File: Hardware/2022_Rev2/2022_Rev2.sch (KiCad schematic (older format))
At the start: 36 parts

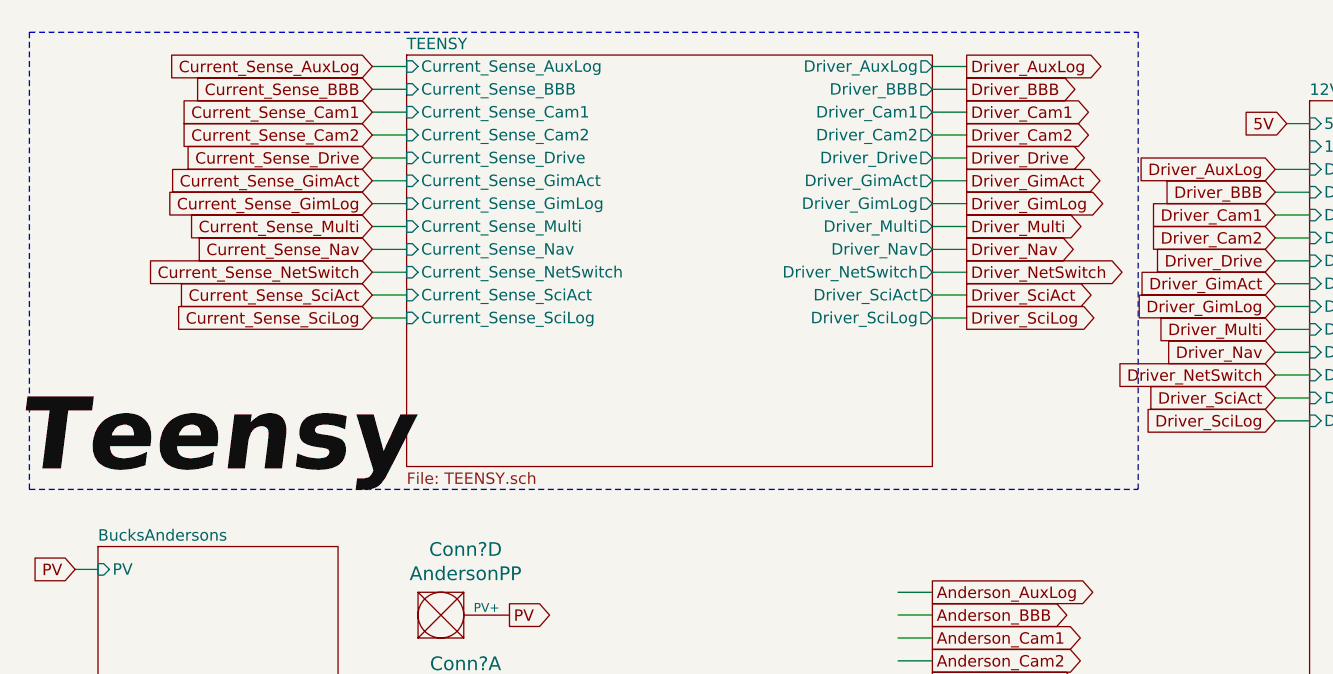
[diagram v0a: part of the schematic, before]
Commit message: molex pins
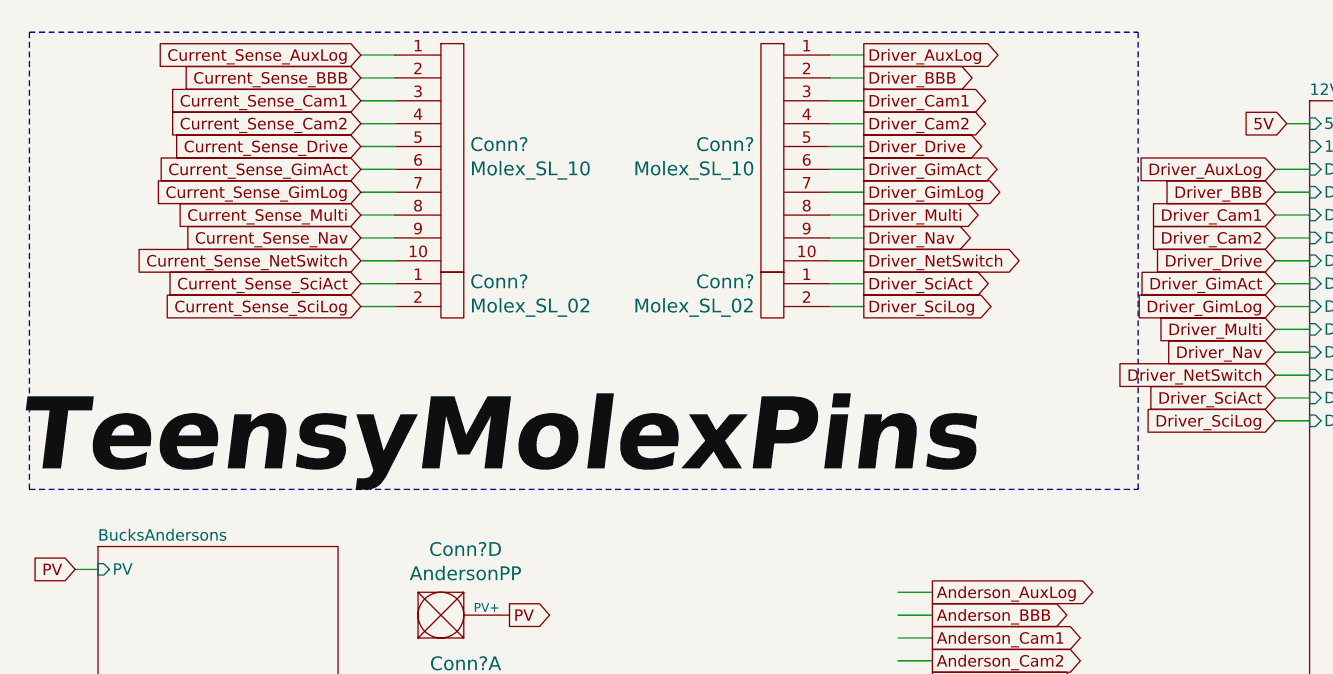
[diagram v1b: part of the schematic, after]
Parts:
- added Conn? (x2): Molex_SL_10, symbol MRDT_Connectors:Molex_SL_10
- added Conn? (x2): Molex_SL_02, symbol MRDT_Connectors:Molex_SL_02
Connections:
- net labels added: TeensyMolexPins
- net labels removed: Teensy
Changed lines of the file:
@@
 $Descr A4 11693 8268
 encoding utf-8
-Sheet 1 5
+Sheet 1 4
 Title ""
 Date ""
@@
 	1    0    0    -1
 $EndComp
-Text GLabel 2000 1050 0    50   Input ~ 0
-Current_Sense_Drive
-Text GLabel 2000 1450 0    50   Input ~ 0
-Current_Sense_Nav
-Wire Wire Line
-	2000 1050 2150 1050
-Wire Wire Line
-	2150 1450 2000 1450
-Text GLabel 4600 1050 2    50   Output ~ 0
-Driver_Drive
-Wire Wire Line
-	4450 1050 4600 1050
-Text GLabel 4600 1450 2    50   Output ~ 0
-Driver_Nav
-Wire Wire Line
-	4450 1450 4600 1450
 Wire Notes Line
 	500  500  5350 500
 Text Label 450  2500 0    315  Italic 63
-Teensy
+TeensyMolexPins
 Wire Notes Line
 	500  2500 5350 2500
@@
 Text Label 7100 7050 0    157  Italic 31
 "Rev4"
-$Sheet
-S 2150 600  2300 1800
-U 62118F7B
-F0 "TEENSY" 50
-F1 "TEENSY.sch" 50
-F2 "Current_Sense_Drive" I L 2150 1050 50
-F3 "Current_Sense_Nav" I L 2150 1450 50
-F4 "Driver_Drive" O R 4450 1050 50
-F5 "Driver_Nav" O R 4450 1450 50
-F6 "Current_Sense_BBB" I L 2150 750 50
-F7 "Current_Sense_Multi" I L 2150 1350 50
-F8 "Current_Sense_Cam2" I L 2150 950 50
-F9 "Current_Sense_Cam1" I L 2150 850 50
-F10 "Driver_BBB" O R 4450 750 50
-F11 "Driver_Multi" O R 4450 1350 50
-F12 "Driver_GimAct" O R 4450 1150 50
-F13 "Driver_Cam1" O R 4450 850 50
-F14 "Driver_Cam2" O R 4450 950 50
-F15 "Current_Sense_GimAct" I L 2150 1150 50
-F16 "Driver_GimLog" O R 4450 1250 50
-F17 "Driver_NetSwitch" O R 4450 1550 50
-F18 "Driver_AuxLog" O R 4450 650 50
-F19 "Driver_SciLog" O R 4450 1750 50
-F20 "Driver_SciAct" O R 4450 1650 50
-F21 "Current_Sense_GimLog" I L 2150 1250 50
-F22 "Current_Sense_NetSwitch" I L 2150 1550 50
-F23 "Current_Sense_SciAct" I L 2150 1650 50
-F24 "Current_Sense_SciLog" I L 2150 1750 50
-F25 "Current_Sense_AuxLog" I L 2150 650 50
-$EndSheet
-Text GLabel 2000 650  0    50   Input ~ 0
-Current_Sense_AuxLog
-Wire Wire Line
-	2000 650  2150 650
-Text GLabel 2000 750  0    50   Input ~ 0
-Current_Sense_BBB
-Wire Wire Line
-	2000 750  2150 750
-Text GLabel 2000 850  0    50   Input ~ 0
-Current_Sense_Cam1
-Wire Wire Line
-	2000 850  2150 850
-Text GLabel 2000 950  0    50   Input ~ 0
-Current_Sense_Cam2
-Wire Wire Line
-	2000 950  2150 950
-Text GLabel 2000 1150 0    50   Input ~ 0
-Current_Sense_GimAct
-Wire Wire Line
-	2000 1150 2150 1150
-Text GLabel 2000 1250 0    50   Input ~ 0
-Current_Sense_GimLog
-Wire Wire Line
-	2000 1250 2150 1250
-Text GLabel 2000 1350 0    50   Input ~ 0
-Current_Sense_Multi
-Wire Wire Line
-	2000 1350 2150 1350
-Text GLabel 2000 1550 0    50   Input ~ 0
-Current_Sense_NetSwitch
-Wire Wire Line
-	2000 1550 2150 1550
-Text GLabel 2000 1650 0    50   Input ~ 0
-Current_Sense_SciAct
-Wire Wire Line
-	2000 1650 2150 1650
-Text GLabel 2000 1750 0    50   Input ~ 0
-Current_Sense_SciLog
-Wire Wire Line
-	2000 1750 2150 1750
-Text GLabel 4600 650  2    50   Output ~ 0
-Driver_AuxLog
-Wire Wire Line
-	4450 650  4600 650
-Text GLabel 4600 750  2    50   Output ~ 0
-Driver_BBB
-Wire Wire Line
-	4450 750  4600 750
-Text GLabel 4600 850  2    50   Output ~ 0
-Driver_Cam1
-Wire Wire Line
-	4450 850  4600 850
-Text GLabel 4600 950  2    50   Output ~ 0
-Driver_Cam2
-Wire Wire Line
-	4450 950  4600 950
-Text GLabel 4600 1150 2    50   Output ~ 0
-Driver_GimAct
-Wire Wire Line
-	4450 1150 4600 1150
-Text GLabel 4600 1250 2    50   Output ~ 0
-Driver_GimLog
-Wire Wire Line
-	4450 1250 4600 1250
-Text GLabel 4600 1350 2    50   Output ~ 0
-Driver_Multi
-Wire Wire Line
-	4450 1350 4600 1350
-Text GLabel 4600 1550 2    50   Output ~ 0
-Driver_NetSwitch
-Wire Wire Line
-	4450 1550 4600 1550
-Text GLabel 4600 1650 2    50   Output ~ 0
-Driver_SciAct
-Wire Wire Line
-	4450 1650 4600 1650
-Text GLabel 4600 1750 2    50   Output ~ 0
-Driver_SciLog
-Wire Wire Line
-	4450 1750 4600 1750
 Text GLabel 5950 1500 0    50   Input ~ 0
 Driver_Drive
@@
 Connection ~ 10150 6500
 Connection ~ 10400 6500
+$Comp
+L MRDT_Connectors:Molex_SL_10 Conn?
+U 1 1 622C6D4E
+P 2300 1550
+F 0 "Conn?" H 2428 2108 60  0000 L CNN
+F 1 "Molex_SL_10" H 2428 2002 60  0000 L CNN
+F 2 "" H 2300 2050 60  0001 C CNN
+F 3 "" H 2300 2050 60  0001 C CNN
+	1    2300 1550
+	1    0    0    -1
+$EndComp
+$Comp
+L MRDT_Connectors:Molex_SL_02 Conn?
+U 1 1 622C7AC7
+P 2300 1750
+F 0 "Conn?" H 2428 1908 60  0000 L CNN
+F 1 "Molex_SL_02" H 2428 1802 60  0000 L CNN
+F 2 "" H 2300 1650 60  0001 C CNN
+F 3 "" H 2300 1650 60  0001 C CNN
+	1    2300 1750
+	1    0    0    -1
+$EndComp
+$Comp
+L MRDT_Connectors:Molex_SL_10 Conn?
+U 1 1 622C9F32
+P 3800 1550
+F 0 "Conn?" H 3928 2108 60  0000 L CNN
+F 1 "Molex_SL_10" H 3928 2002 60  0000 L CNN
+F 2 "" H 3800 2050 60  0001 C CNN
+F 3 "" H 3800 2050 60  0001 C CNN
+	1    3800 1550
+	-1   0    0    -1
+$EndComp
+$Comp
+L MRDT_Connectors:Molex_SL_02 Conn?
+U 1 1 622C9F38
+P 3800 1750
+F 0 "Conn?" H 3928 1908 60  0000 L CNN
+F 1 "Molex_SL_02" H 3928 1802 60  0000 L CNN
+F 2 "" H 3800 1650 60  0001 C CNN
+F 3 "" H 3800 1650 60  0001 C CNN
+	1    3800 1750
+	-1   0    0    -1
+$EndComp
+Text GLabel 1950 1000 0    50   Input ~ 0
+Current_Sense_Drive
+Text GLabel 1950 1400 0    50   Input ~ 0
+Current_Sense_Nav
+Wire Wire Line
+	1950 1000 2100 1000
+Wire Wire Line
+	2100 1400 1950 1400
+Text GLabel 1950 600  0    50   Input ~ 0
+Current_Sense_AuxLog
+Wire Wire Line
+	1950 600  2100 600
+Text GLabel 1950 700  0    50   Input ~ 0
+Current_Sense_BBB
+Wire Wire Line
+	1950 700  2100 700
+Text GLabel 1950 800  0    50   Input ~ 0
+Current_Sense_Cam1
+Wire Wire Line
+	1950 800  2100 800
+Text GLabel 1950 900  0    50   Input ~ 0
+Current_Sense_Cam2
+Wire Wire Line
+	1950 900  2100 900
+Text GLabel 1950 1100 0    50   Input ~ 0
+Current_Sense_GimAct
+Wire Wire Line
+	1950 1100 2100 1100
+Text GLabel 1950 1200 0    50   Input ~ 0
+Current_Sense_GimLog
+Wire Wire Line
+	1950 1200 2100 1200
+Text GLabel 1950 1300 0    50   Input ~ 0
+Current_Sense_Multi
+Wire Wire Line
+	1950 1300 2100 1300
+Text GLabel 1950 1500 0    50   Input ~ 0
+Current_Sense_NetSwitch
+Wire Wire Line
+	1950 1500 2100 1500
+Text GLabel 1950 1600 0    50   Input ~ 0
+Current_Sense_SciAct
+Wire Wire Line
+	1950 1600 2100 1600
+Text GLabel 1950 1700 0    50   Input ~ 0
+Current_Sense_SciLog
+Wire Wire Line
+	1950 1700 2100 1700
+Text GLabel 4150 1000 2    50   Output ~ 0
+Driver_Drive
+Wire Wire Line
+	4000 1000 4150 1000
+Text GLabel 4150 1400 2    50   Output ~ 0
+Driver_Nav
+Wire Wire Line
+	4000 1400 4150 1400
+Text GLabel 4150 600  2    50   Output ~ 0
+Driver_AuxLog
+Wire Wire Line
+	4000 600  4150 600
+Text GLabel 4150 700  2    50   Output ~ 0
+Driver_BBB
+Wire Wire Line
+	4000 700  4150 700
+Text GLabel 4150 800  2    50   Output ~ 0
+Driver_Cam1
+Wire Wire Line
+	4000 800  4150 800
+Text GLabel 4150 900  2    50   Output ~ 0
+Driver_Cam2
+Wire Wire Line
+	4000 900  4150 900
+Text GLabel 4150 1100 2    50   Output ~ 0
+Driver_GimAct
+Wire Wire Line
+	4000 1100 4150 1100
+Text GLabel 4150 1200 2    50   Output ~ 0
+Driver_GimLog
+Wire Wire Line
+	4000 1200 4150 1200
+Text GLabel 4150 1300 2    50   Output ~ 0
+Driver_Multi
+Wire Wire Line
+	4000 1300 4150 1300
+Text GLabel 4150 1500 2    50   Output ~ 0
+Driver_NetSwitch
+Wire Wire Line
+	4000 1500 4150 1500
+Text GLabel 4150 1600 2    50   Output ~ 0
+Driver_SciAct
+Wire Wire Line
+	4000 1600 4150 1600
+Text GLabel 4150 1700 2    50   Output ~ 0
+Driver_SciLog
+Wire Wire Line
+	4000 1700 4150 1700
 $EndSCHEMATC
